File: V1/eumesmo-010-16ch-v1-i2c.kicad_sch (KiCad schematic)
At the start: 132 parts, among them U10 MCP23017, U13 ISO1540, U14 LM324, U15 LM324, U16 LM324, U17 LM324, U8 PCA9685PW

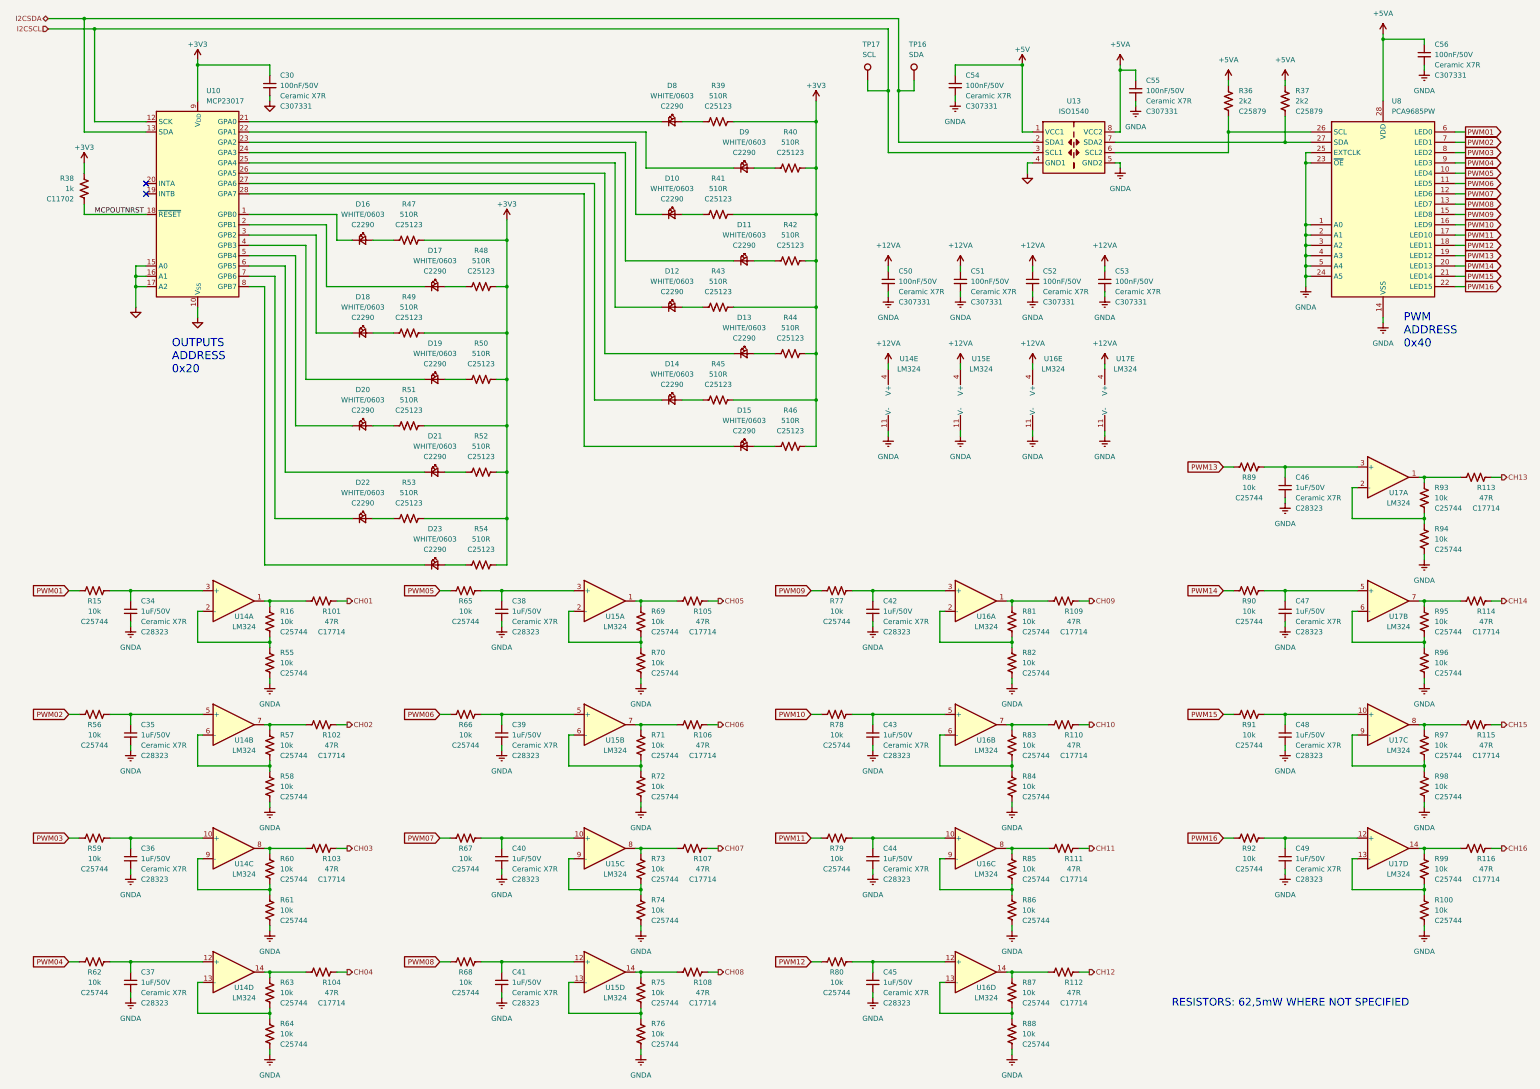
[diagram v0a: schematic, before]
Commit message: Development
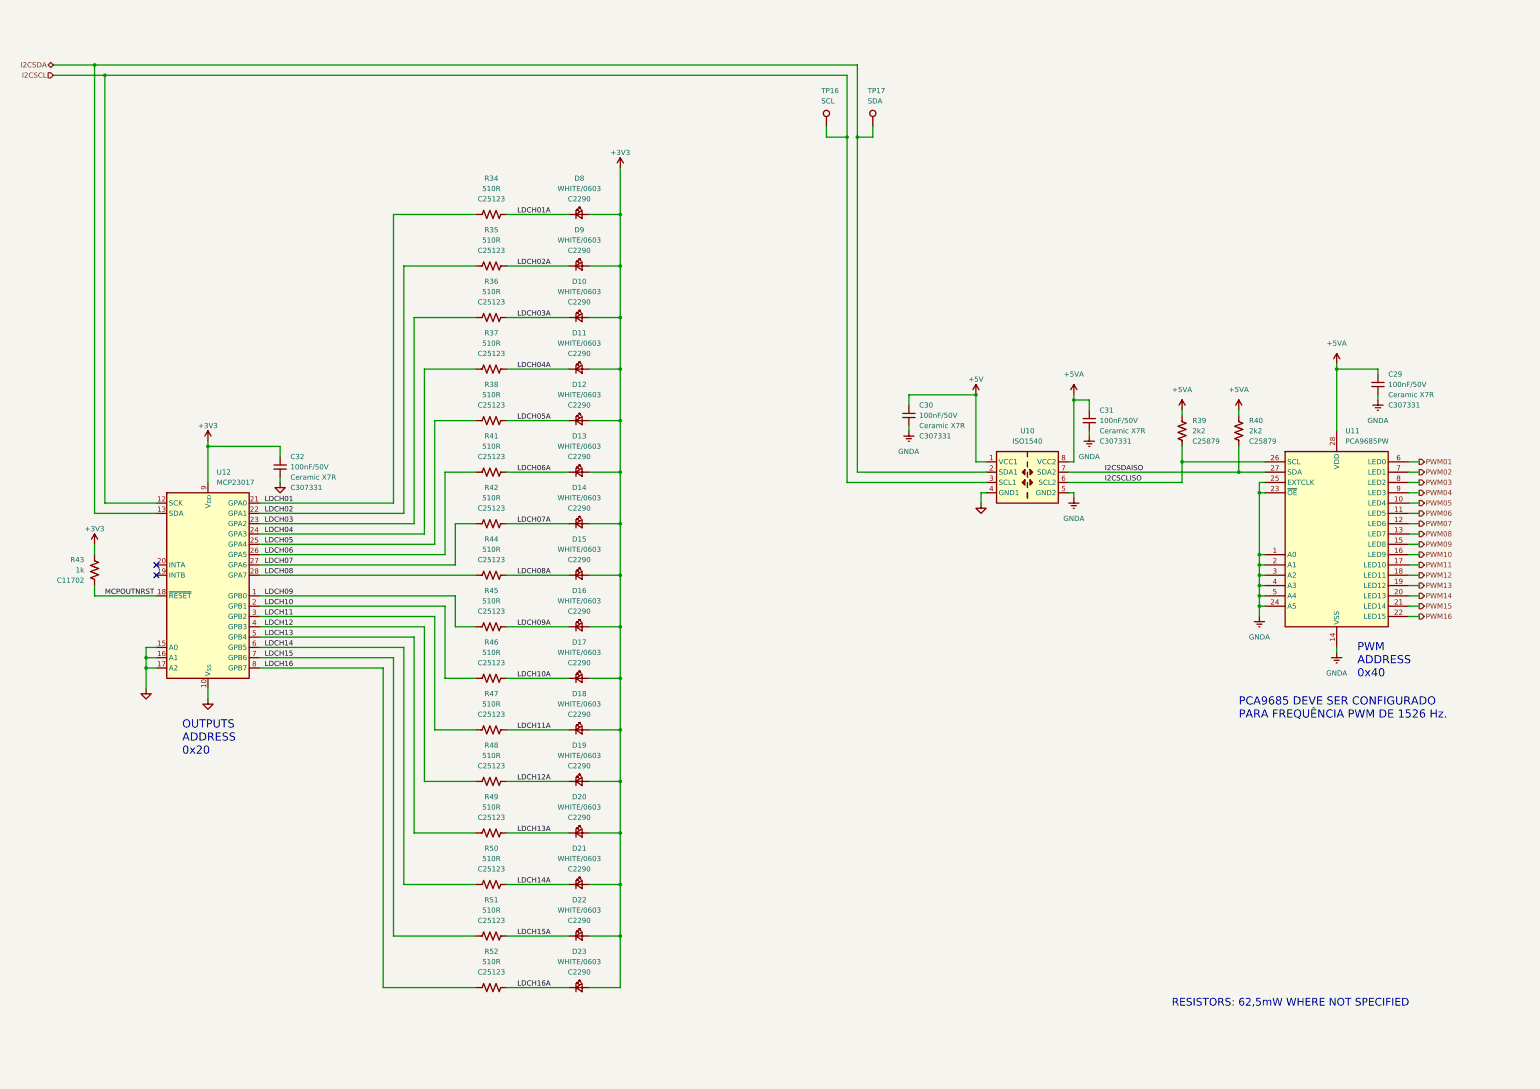
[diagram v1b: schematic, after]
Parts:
- removed C34, C35, C36, C37, C38, C39, C40, C41, C42, C43, C44, C45, C46, C47, C48, C49: 1uF/50V, Tales:C_0805_2012Metric, symbol Device:C_Small
- removed C50, C51, C52, C53: 100nF/50V, Tales:C_0402_1005Metric, symbol Device:C_Small
- removed R100, R15, R16, R55, R56, R57, R58, R59, R60, R61, R62, R63, R64, R65, R66, R67, R68, R69, R70, R71, R72, R73, R74, R75, R76, R77, R78, R79, R80, R81, R82, R83, R84, R85, R86, R87, R88, R89, R90, R91, R92, R93, R94, R95, R96, R97, R98, R99: 10k, Tales:R_0402_1005Metric, symbol Device:R_US
- removed R101, R102, R103, R104, R105, R106, R107, R108, R109, R110, R111, R112, R113, R114, R115, R116: 47R, Tales:R_0805_2012Metric, symbol Device:R_US
- removed U14, U15, U16, U17: LM324, symbol Amplifier_Operational:LM324
- D10, D11, D12, D13, D14, D15, D16, D17, D18, D19, D20, D21, D22, D23, D8, D9: Technology (none) -> LED
- U10: renamed from U13; Case (none) -> SOIC-8; JLCPCB BOM (none) -> 1; LCSC Part # (none) -> C179739; Mfr (none) -> Texas Instruments; Mfr PN (none) -> ISO1540DR; Technology (none) -> I2C Isolator; Vendor (none) -> JLCPCB; Vendor PN (none) -> C179739
- U11: renamed from U8; Case (none) -> TSSOP-28; JLCPCB BOM (none) -> 1; LCSC Part # (none) -> C2678753; Mfr (none) -> NXP; Mfr PN (none) -> PCA9685PW; Vendor (none) -> JLCPCB; Vendor PN (none) -> C2678753
- renumbered C56 to C29, C54 to C30, C55 to C31, C30 to C32, R39 to R34, R40 to R35, R41 to R36, R42 to R37, R43 to R38, R36 to R39, R37 to R40, R44 to R41, R45 to R42, R38 to R43, R46 to R44, R47 to R45, R48 to R46, R49 to R47, R50 to R48, R51 to R49, R52 to R50, R53 to R51, R54 to R52, TP17 to TP16, TP16 to TP17, U10 to U12
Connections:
- net +3V3: now also D10.2 (A), D11.2 (A), D12.2 (A), D13.2 (A), D14.2 (A), D15.2 (A), D16.2 (A), D17.2 (A), D18.2 (A), D19.2 (A), D20.2 (A), D21.2 (A), D22.2 (A), D23.2 (A), D8.2 (A), D9.2 (A); no longer R34.2, R35.2, R36.2, R37.2, R38.2, R41.2, R42.2, R44.2, R45.2, R46.2, R47.2, R48.2, R49.2, R50.2, R51.2, R52.2
- net LDCH03: now reaches R36.1
- net LDCH03: now also U12.23 (GPA2); no longer D10.2 (A)
- net LDCH02: now reaches U12.22 (GPA1)
- net LDCH02: now also R35.1; no longer D9.1 (K)
- net LDCH06: now reaches U12.26 (GPA5)
- net LDCH06: now also R41.1; no longer D13.1 (K)
- net LDCH12: now reaches R48.1
- net LDCH12: now also U12.4 (GPB3); no longer D19.2 (A)
- net LDCH16: now reaches U12.8 (GPB7)
- net LDCH16: now also R52.1; no longer D23.1 (K)
- net LDCH15: now reaches R51.1
- net LDCH15: now also U12.7 (GPB6); no longer D22.2 (A)
- net LDCH15A: now reaches D22.1 (K)
- net LDCH15A: now also R51.2; no longer U12.7 (GPB6)
- net LDCH05: now reaches R38.1
- net LDCH05: now also U12.25 (GPA4); no longer D12.2 (A)
- net LDCH04: now reaches R37.1
- net LDCH04: now also U12.24 (GPA3); no longer D11.2 (A)
- net LDCH10: now reaches U12.2 (GPB1)
- net LDCH10: now also R46.1; no longer D17.1 (K)
- net LDCH09: now reaches R45.1
- net LDCH09: now also U12.1 (GPB0); no longer D16.2 (A)
- net LDCH13: now reaches U12.5 (GPB4)
- net LDCH13: now also R49.1; no longer D20.1 (K)
- net LDCH01: now reaches U12.21 (GPA0)
- net LDCH01: now also R34.1; no longer D8.1 (K)
- net LDCH07: now reaches R42.1
- net LDCH07: now also U12.27 (GPA6); no longer D14.2 (A)
- net LDCH03A: now reaches D10.1 (K)
- net LDCH03A: now also R36.2; no longer U12.23 (GPA2)
- net LDCH11: now reaches U12.3 (GPB2)
- net LDCH11: now also R47.1; no longer D18.1 (K)
- net I2CSCLISO: now reaches R39.2, U10.6 (SCL2), U11.26 (SCL)
- net I2CSDAISO: now reaches R40.2, U10.7 (SDA2), U11.27 (SDA)
- net LDCH08: now reaches U12.28 (GPA7)
- net LDCH08: now also R44.1; no longer D15.1 (K)
- net LDCH14: now reaches R50.1
- net LDCH14: now also U12.6 (GPB5); no longer D21.2 (A)
- net LDCH04A: now reaches D11.1 (K)
- net LDCH04A: now also R37.2; no longer U12.24 (GPA3)
- net LDCH09A: now reaches D16.1 (K)
- net LDCH09A: now also R45.2; no longer U12.1 (GPB0)
- net LDCH05A: now reaches D12.1 (K)
- net LDCH05A: now also R38.2; no longer U12.25 (GPA4)
- net LDCH07A: now reaches D14.1 (K)
- net LDCH07A: now also R42.2; no longer U12.27 (GPA6)
- net LDCH12A: now reaches D19.1 (K)
- net LDCH12A: now also R48.2; no longer U12.4 (GPB3)
- net LDCH14A: now reaches D21.1 (K)
- net LDCH14A: now also R50.2; no longer U12.6 (GPB5)
- new net LDCH01A: D8.1 (K), R34.2
- new net LDCH02A: D9.1 (K), R35.2
- new net LDCH06A: D13.1 (K), R41.2
- new net LDCH08A: D15.1 (K), R44.2
- new net LDCH10A: D17.1 (K), R46.2
- new net LDCH11A: D18.1 (K), R47.2
- new net LDCH13A: D20.1 (K), R49.2
- new net LDCH16A: D23.1 (K), R52.2
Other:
- note added: "PCA9685 DEVE SER CONFIGURADO PARA FREQUÊNCIA PWM DE 1526 Hz."
- moved on the sheet: C29, C30, C31, C32, D10, D11, D12, D13, D14, D15, D16, D17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
